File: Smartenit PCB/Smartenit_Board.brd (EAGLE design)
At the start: 55.3 x 72.5 mm, 85 parts, among them J3 2X5CONNECTOR1.27MM, Q1 QUARTZ_3.58M_2PIN, U1 ADE7953, U2 ESP-WROOM-32, U3 SN74LVC1G3157

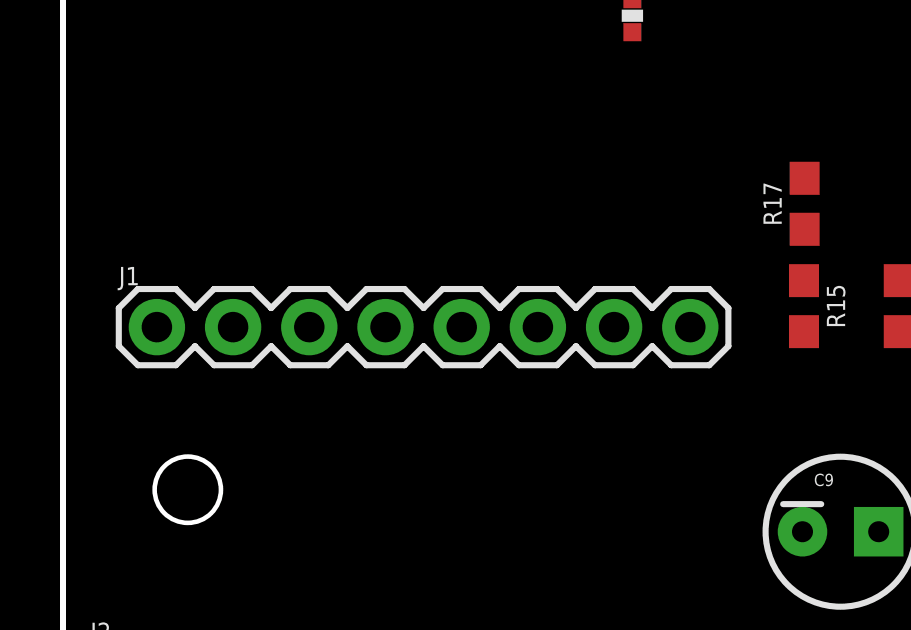
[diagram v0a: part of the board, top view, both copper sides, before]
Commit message: no error still
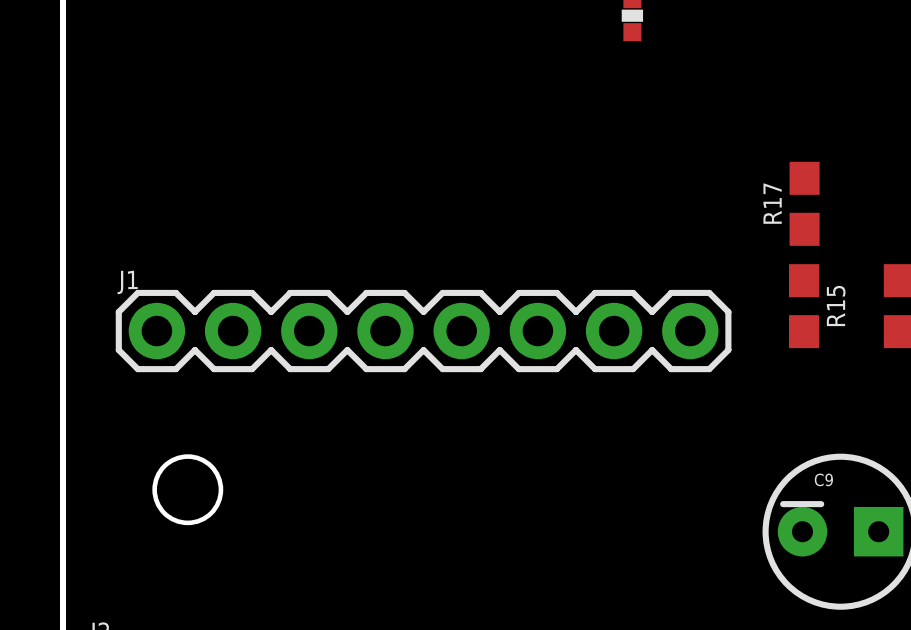
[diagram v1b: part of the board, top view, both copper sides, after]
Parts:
- moved J1 0.13 mm to (3.13, -56.5)
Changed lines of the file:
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@@
 <element name="C4" library="Nizanlib" package="0402-CAP" value="104n" x="8.35" y="-34.61"/>
 <element name="C9" library="SparkFun" package="CPOL-RADIAL-10UF-25V" value="" x="25.92" y="-63.2"/>
-<element name="J1" library="SparkFun-Connectors" package="1X08" value="" x="3.13" y="-56.38">
-<attribute name="PROD_ID" value="CONN-08438" x="3.13" y="-56.38" size="1.778" layer="27" display="off"/>
+<element name="J1" library="SparkFun-Connectors" package="1X08" value="" x="3.13" y="-56.51">
+<attribute name="PROD_ID" value="CONN-08438" x="3.13" y="-56.51" size="1.778" layer="27" display="off"/>
 </element>
 <element name="J2" library="SparkFun-Connectors" package="1X06" value="" x="2.18" y="-68.24">
@@
 <contactref element="R12" pad="1"/>
 <contactref element="J1" pad="6"/>
-<wire x1="9.41" y1="-39.75" x2="15.83" y2="-56.38" width="0" layer="19" extent="1-1"/>
+<wire x1="9.41" y1="-39.75" x2="15.83" y2="-56.51" width="0" layer="19" extent="1-1"/>
 <wire x1="7.78" y1="-32.3" x2="9.41" y2="-39.75" width="0" layer="19" extent="1-1"/>
 </signal>
@@
 <contactref element="R7" pad="1"/>
 <contactref element="J1" pad="5"/>
-<wire x1="5.35" y1="-39.76" x2="13.29" y2="-56.38" width="0" layer="19" extent="1-1"/>
+<wire x1="5.35" y1="-39.76" x2="13.29" y2="-56.51" width="0" layer="19" extent="1-1"/>
 <wire x1="4.64" y1="-32.3" x2="5.35" y2="-39.76" width="0" layer="19" extent="1-1"/>
 </signal>
@@
 <contactref element="C25" pad="2"/>
 <contactref element="R36" pad="1"/>
-<wire x1="5.67" y1="-56.38" x2="4.72" y2="-68.24" width="0" layer="19" extent="1-1"/>
-<wire x1="18.98" y1="-46.55" x2="5.67" y2="-56.38" width="0" layer="19" extent="1-1"/>
+<wire x1="5.67" y1="-56.51" x2="4.72" y2="-68.24" width="0" layer="19" extent="1-1"/>
+<wire x1="18.98" y1="-46.55" x2="5.67" y2="-56.51" width="0" layer="19" extent="1-1"/>
 <wire x1="17.76" y1="-43.52" x2="18.98" y2="-46.55" width="0" layer="19" extent="1-1"/>
 <wire x1="17.761" y1="-42.344" x2="17.76" y2="-43.52" width="0" layer="19" extent="1-1"/>
@@
 <contactref element="R4" pad="1"/>
 <contactref element="J1" pad="8"/>
-<wire x1="16.66" y1="-43.52" x2="20.91" y2="-56.38" width="0" layer="19" extent="1-1"/>
+<wire x1="16.66" y1="-43.52" x2="20.91" y2="-56.51" width="0" layer="19" extent="1-1"/>
 <wire x1="16.64" y1="-42.33" x2="16.66" y2="-43.52" width="0" layer="19" extent="1-1"/>
 </signal>
@@
 <contactref element="R22" pad="1"/>
 <contactref element="J1" pad="7"/>
-<wire x1="18.98" y1="-45.45" x2="18.37" y2="-56.38" width="0" layer="19" extent="1-1"/>
+<wire x1="18.98" y1="-45.45" x2="18.37" y2="-56.51" width="0" layer="19" extent="1-1"/>
 <wire x1="18.93" y1="-42.37" x2="18.98" y2="-45.45" width="0" layer="19" extent="1-1"/>
 </signal>
@@
 <contactref element="R32" pad="2"/>
 <contactref element="D6" pad="C"/>
-<wire x1="2.93" y1="-17.52" x2="3.13" y2="-56.38" width="0" layer="19" extent="1-1"/>
+<wire x1="2.93" y1="-17.52" x2="3.13" y2="-56.51" width="0" layer="19" extent="1-1"/>
 <wire x1="19.31" y1="-6.75" x2="2.93" y2="-17.52" width="0" layer="19" extent="1-1"/>
 <wire x1="22.26" y1="-5.85" x2="19.31" y2="-6.75" width="0" layer="19" extent="1-1"/>
@@
 <contactref element="J1" pad="3"/>
 <contactref element="R34" pad="1"/>
-<wire x1="25.83" y1="-20.18" x2="8.21" y2="-56.38" width="0" layer="19" extent="1-1"/>
+<wire x1="25.83" y1="-20.18" x2="8.21" y2="-56.51" width="0" layer="19" extent="1-1"/>
 </signal>
 <signal name="LNV1">
 <contactref element="J1" pad="4"/>
 <contactref element="R35" pad="1"/>
-<wire x1="28.52" y1="-19.2" x2="10.75" y2="-56.38" width="0" layer="19" extent="1-1"/>
+<wire x1="28.52" y1="-19.2" x2="10.75" y2="-56.51" width="0" layer="19" extent="1-1"/>
 </signal>
 <signal name="DIO12">

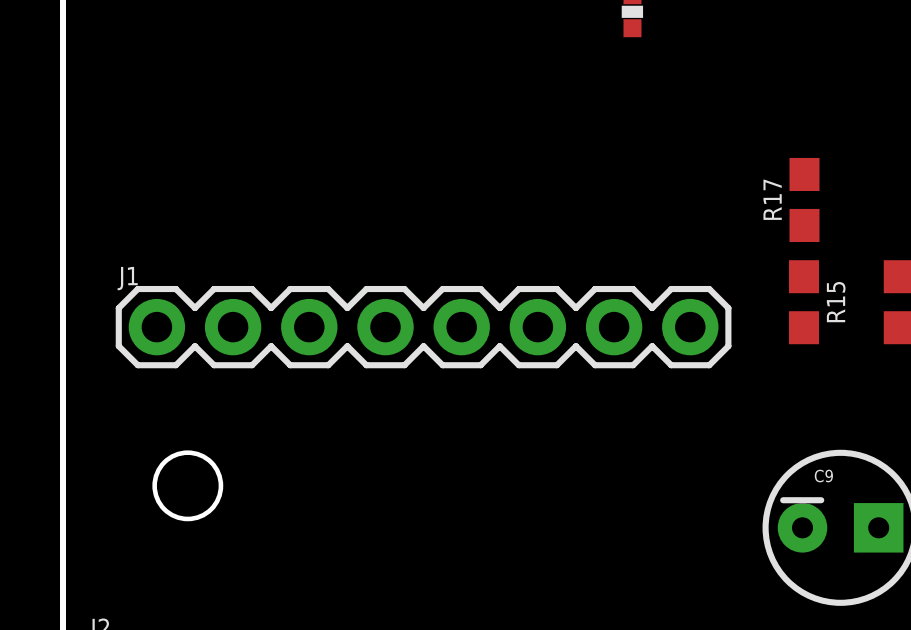
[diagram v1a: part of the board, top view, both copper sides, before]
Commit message: no error
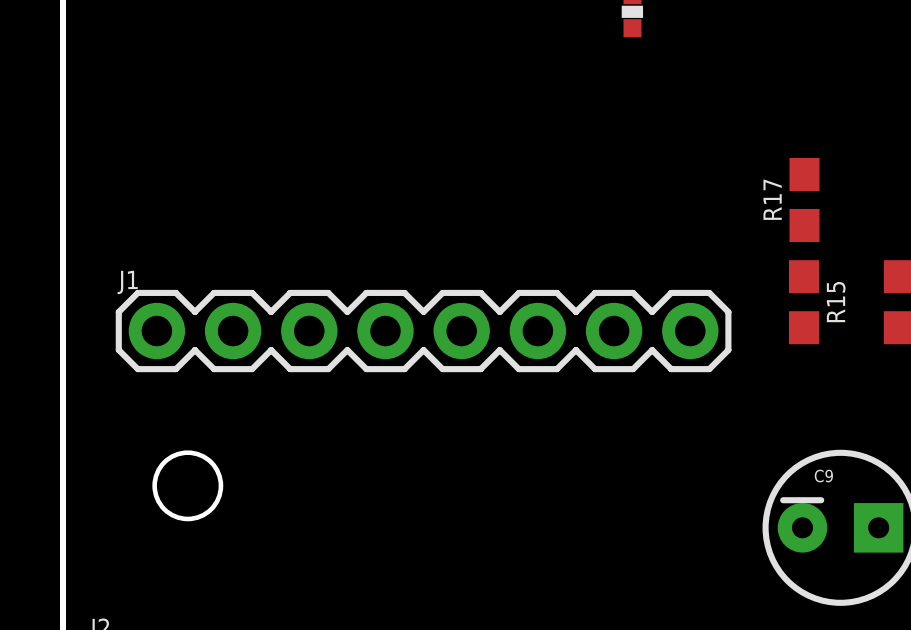
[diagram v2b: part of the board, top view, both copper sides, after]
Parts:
- moved J1 0.13 mm to (3.13, -56.6)
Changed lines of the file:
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@@
 <element name="C4" library="Nizanlib" package="0402-CAP" value="104n" x="8.35" y="-34.61"/>
 <element name="C9" library="SparkFun" package="CPOL-RADIAL-10UF-25V" value="" x="25.92" y="-63.2"/>
-<element name="J1" library="SparkFun-Connectors" package="1X08" value="" x="3.13" y="-56.51">
-<attribute name="PROD_ID" value="CONN-08438" x="3.13" y="-56.51" size="1.778" layer="27" display="off"/>
+<element name="J1" library="SparkFun-Connectors" package="1X08" value="" x="3.13" y="-56.64">
+<attribute name="PROD_ID" value="CONN-08438" x="3.13" y="-56.64" size="1.778" layer="27" display="off"/>
 </element>
 <element name="J2" library="SparkFun-Connectors" package="1X06" value="" x="2.18" y="-68.24">
@@
 <contactref element="R12" pad="1"/>
 <contactref element="J1" pad="6"/>
-<wire x1="9.41" y1="-39.75" x2="15.83" y2="-56.51" width="0" layer="19" extent="1-1"/>
+<wire x1="9.41" y1="-39.75" x2="15.83" y2="-56.64" width="0" layer="19" extent="1-1"/>
 <wire x1="7.78" y1="-32.3" x2="9.41" y2="-39.75" width="0" layer="19" extent="1-1"/>
 </signal>
@@
 <contactref element="R7" pad="1"/>
 <contactref element="J1" pad="5"/>
-<wire x1="5.35" y1="-39.76" x2="13.29" y2="-56.51" width="0" layer="19" extent="1-1"/>
+<wire x1="5.35" y1="-39.76" x2="13.29" y2="-56.64" width="0" layer="19" extent="1-1"/>
 <wire x1="4.64" y1="-32.3" x2="5.35" y2="-39.76" width="0" layer="19" extent="1-1"/>
 </signal>
@@
 <contactref element="C25" pad="2"/>
 <contactref element="R36" pad="1"/>
-<wire x1="5.67" y1="-56.51" x2="4.72" y2="-68.24" width="0" layer="19" extent="1-1"/>
-<wire x1="18.98" y1="-46.55" x2="5.67" y2="-56.51" width="0" layer="19" extent="1-1"/>
+<wire x1="5.67" y1="-56.64" x2="4.72" y2="-68.24" width="0" layer="19" extent="1-1"/>
+<wire x1="18.98" y1="-46.55" x2="5.67" y2="-56.64" width="0" layer="19" extent="1-1"/>
 <wire x1="17.76" y1="-43.52" x2="18.98" y2="-46.55" width="0" layer="19" extent="1-1"/>
 <wire x1="17.761" y1="-42.344" x2="17.76" y2="-43.52" width="0" layer="19" extent="1-1"/>
@@
 <contactref element="R4" pad="1"/>
 <contactref element="J1" pad="8"/>
-<wire x1="16.66" y1="-43.52" x2="20.91" y2="-56.51" width="0" layer="19" extent="1-1"/>
+<wire x1="16.66" y1="-43.52" x2="20.91" y2="-56.64" width="0" layer="19" extent="1-1"/>
 <wire x1="16.64" y1="-42.33" x2="16.66" y2="-43.52" width="0" layer="19" extent="1-1"/>
 </signal>
@@
 <contactref element="R22" pad="1"/>
 <contactref element="J1" pad="7"/>
-<wire x1="18.98" y1="-45.45" x2="18.37" y2="-56.51" width="0" layer="19" extent="1-1"/>
+<wire x1="18.98" y1="-45.45" x2="18.37" y2="-56.64" width="0" layer="19" extent="1-1"/>
 <wire x1="18.93" y1="-42.37" x2="18.98" y2="-45.45" width="0" layer="19" extent="1-1"/>
 </signal>
@@
 <contactref element="R32" pad="2"/>
 <contactref element="D6" pad="C"/>
-<wire x1="2.93" y1="-17.52" x2="3.13" y2="-56.51" width="0" layer="19" extent="1-1"/>
+<wire x1="2.93" y1="-17.52" x2="3.13" y2="-56.64" width="0" layer="19" extent="1-1"/>
 <wire x1="19.31" y1="-6.75" x2="2.93" y2="-17.52" width="0" layer="19" extent="1-1"/>
 <wire x1="22.26" y1="-5.85" x2="19.31" y2="-6.75" width="0" layer="19" extent="1-1"/>
@@
 <contactref element="J1" pad="3"/>
 <contactref element="R34" pad="1"/>
-<wire x1="25.83" y1="-20.18" x2="8.21" y2="-56.51" width="0" layer="19" extent="1-1"/>
+<wire x1="25.83" y1="-20.18" x2="8.21" y2="-56.64" width="0" layer="19" extent="1-1"/>
 </signal>
 <signal name="LNV1">
 <contactref element="J1" pad="4"/>
 <contactref element="R35" pad="1"/>
-<wire x1="28.52" y1="-19.2" x2="10.75" y2="-56.51" width="0" layer="19" extent="1-1"/>
+<wire x1="28.52" y1="-19.2" x2="10.75" y2="-56.64" width="0" layer="19" extent="1-1"/>
 </signal>
 <signal name="DIO12">
